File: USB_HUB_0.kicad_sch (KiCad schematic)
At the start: 30 parts, among them U1 VL822-QFN76, U2 W25Q32JVZPIQ, Y1 25Mhz

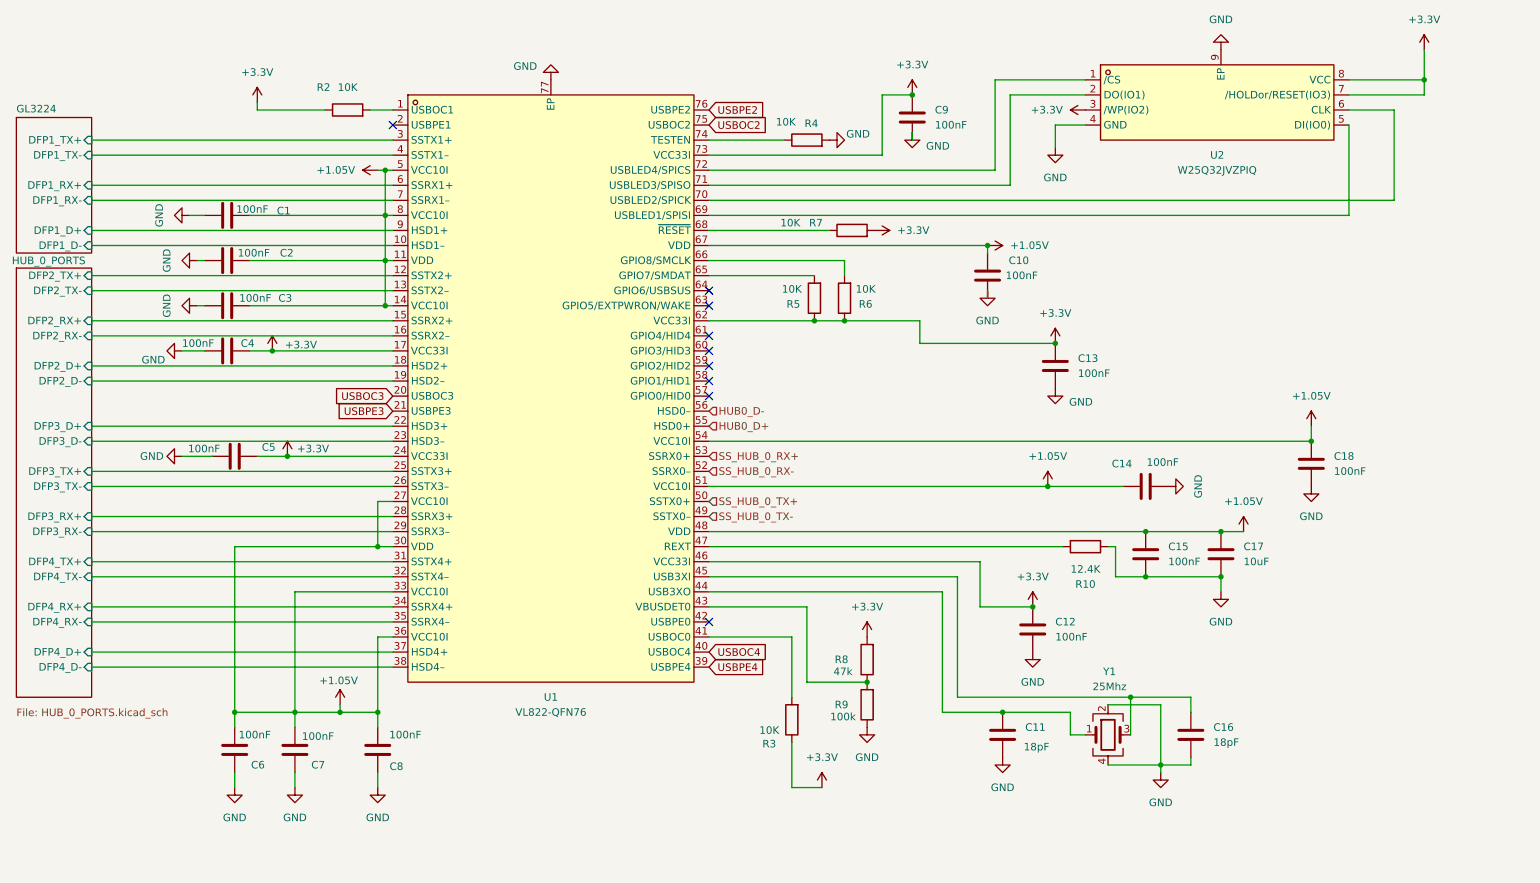
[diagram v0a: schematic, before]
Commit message: .
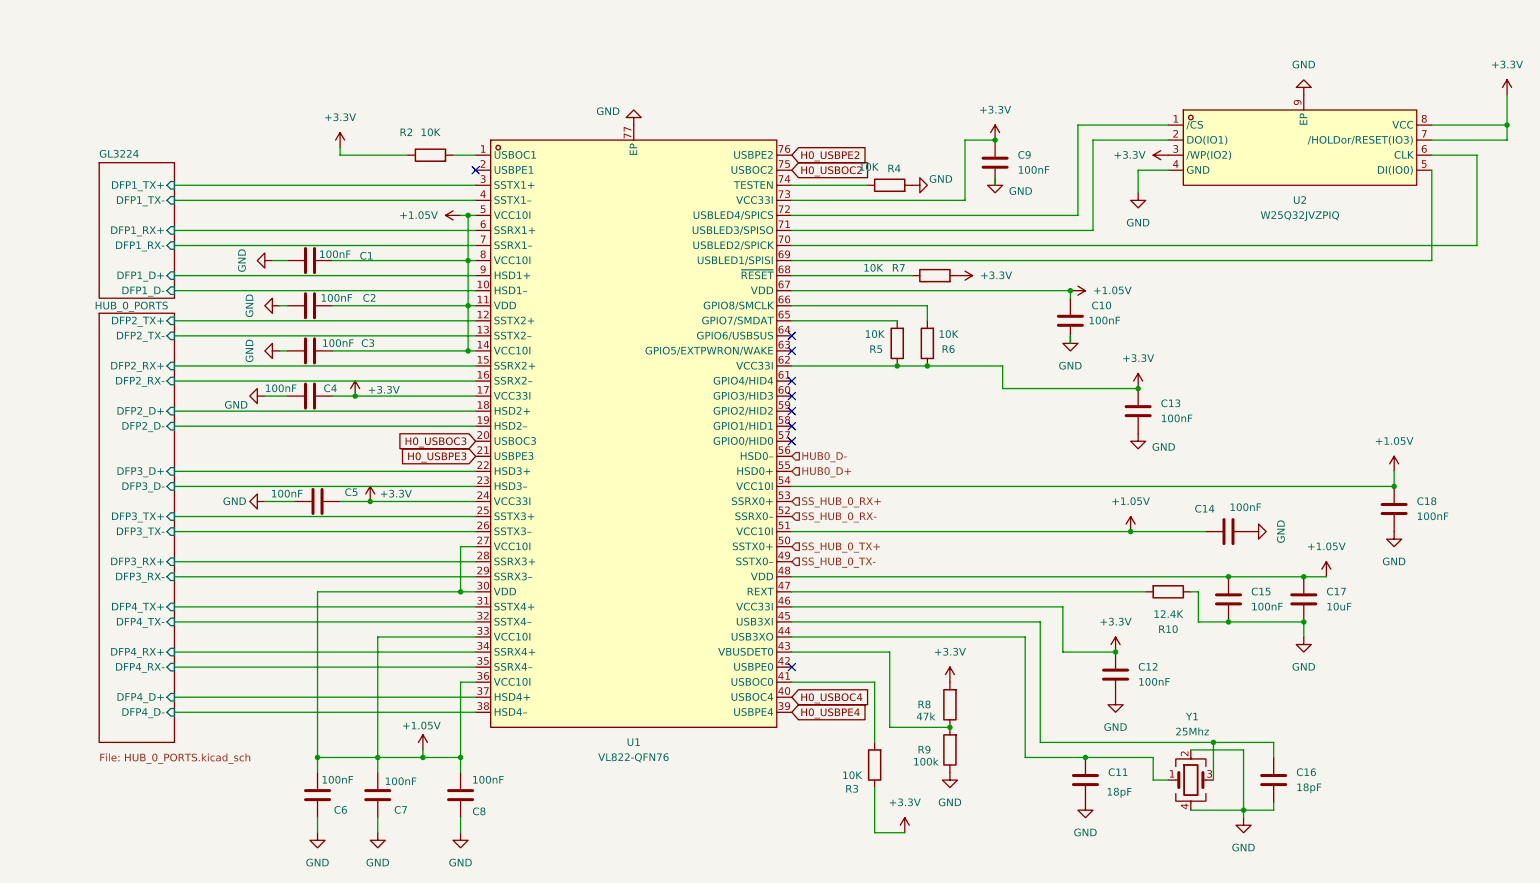
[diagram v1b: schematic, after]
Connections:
- net USBOC2 renamed H0_USBOC2
- net USBOC3 renamed H0_USBOC3
- net USBOC4 renamed H0_USBOC4
- net USBPE2 renamed H0_USBPE2
- net USBPE3 renamed H0_USBPE3
- net USBPE4 renamed H0_USBPE4
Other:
- moved on the sheet: C1, C10, C11, C12, C13, C14, C15, C16, C17, C18, C2, C3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
